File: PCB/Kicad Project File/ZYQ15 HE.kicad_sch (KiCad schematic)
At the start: 130 parts, among them J1 I2C OLED, U16 ESP32-S3-DevKitC

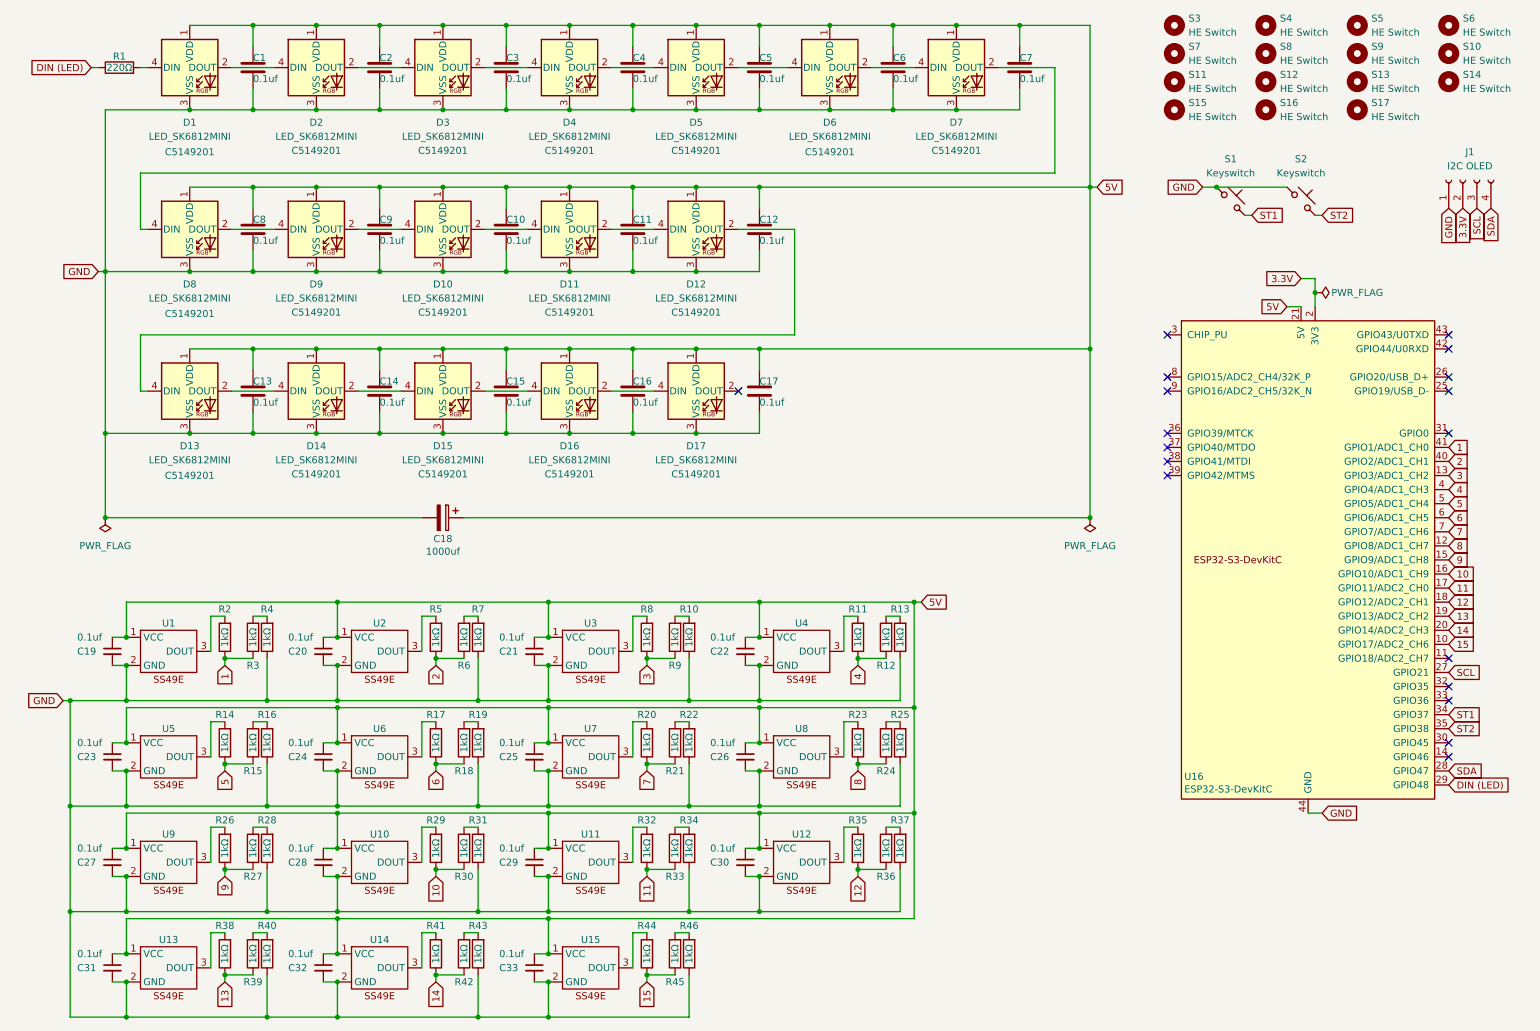
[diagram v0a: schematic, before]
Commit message: Updated PCB design files
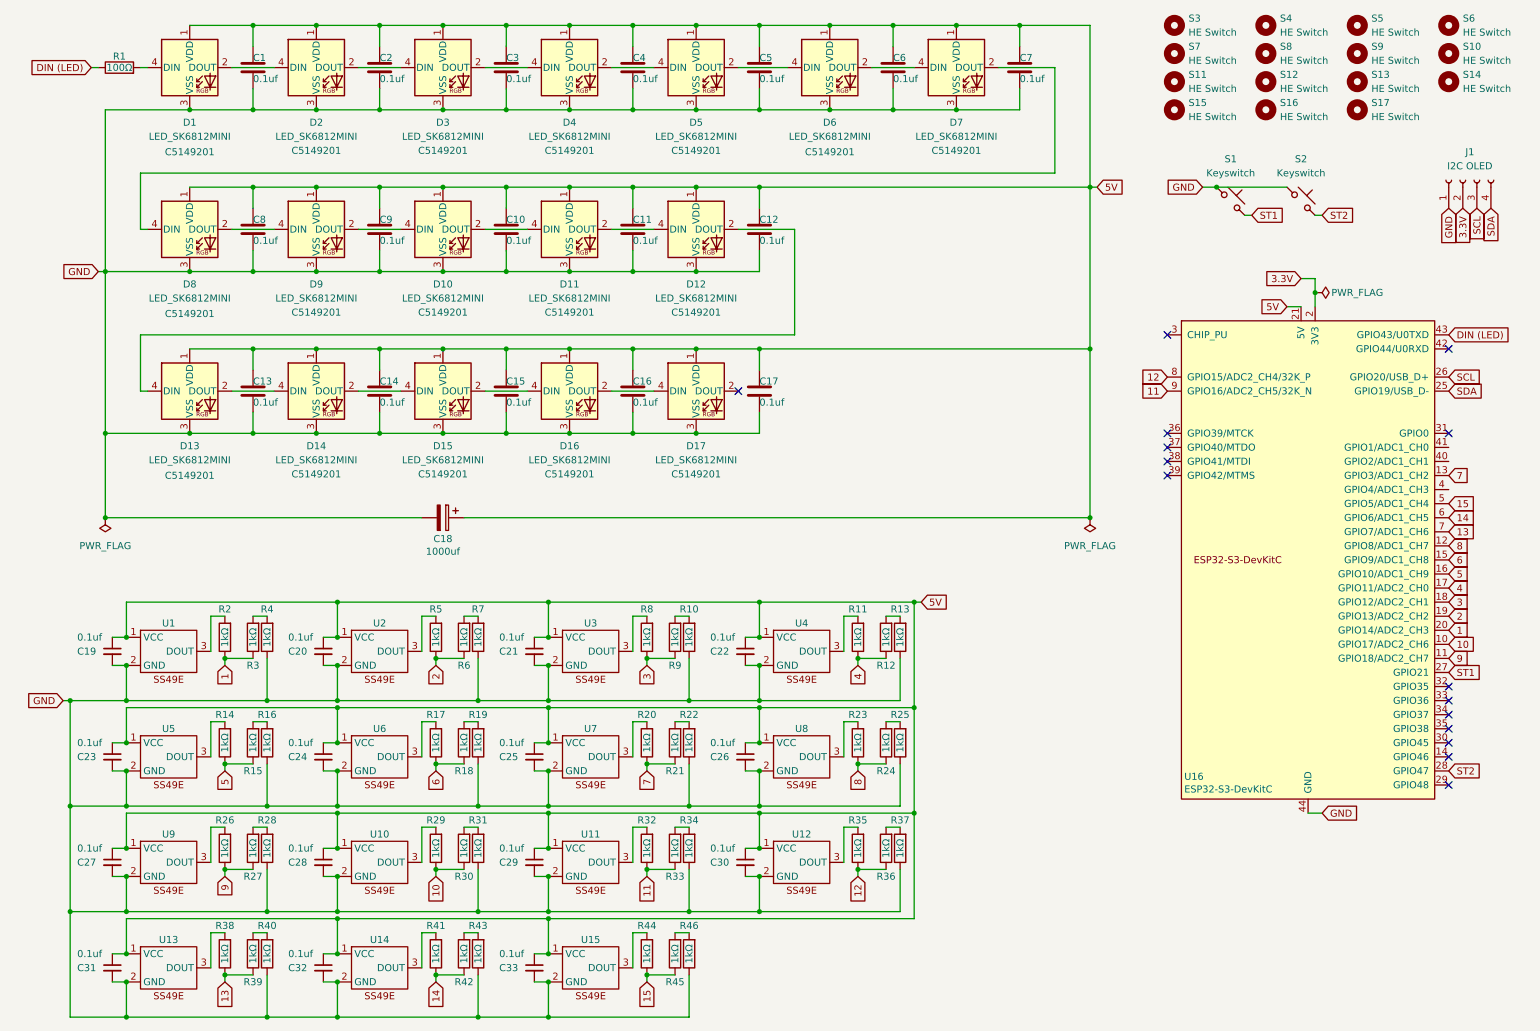
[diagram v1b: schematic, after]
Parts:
- C18: footprint Capacitor_THT:CP_Radial_D10.0mm_P5.00mm -> Capacitor_THT:CP_Radial_D10.0mm_P5.00mm_BACK
- R1: value 220Ω -> 100Ω
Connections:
- net 1: now also U16.20 (GPIO14/ADC2_CH3); no longer U16.41 (GPIO1/ADC1_CH0)
- net 10: now also U16.10 (GPIO17/ADC2_CH6); no longer U16.16 (GPIO10/ADC1_CH9)
- net 11: now also U16.9 (GPIO16/ADC2_CH5/32K_N); no longer U16.17 (GPIO11/ADC2_CH0)
- net 12: now also U16.8 (GPIO15/ADC2_CH4/32K_P); no longer U16.18 (GPIO12/ADC2_CH1)
- net 13: now also U16.7 (GPIO7/ADC1_CH6); no longer U16.19 (GPIO13/ADC2_CH2)
- net 14: now also U16.6 (GPIO6/ADC1_CH5); no longer U16.20 (GPIO14/ADC2_CH3)
- net 15: now also U16.5 (GPIO5/ADC1_CH4); no longer U16.10 (GPIO17/ADC2_CH6)
- net 2: now also U16.19 (GPIO13/ADC2_CH2); no longer U16.40 (GPIO2/ADC1_CH1)
- net 3: now also U16.18 (GPIO12/ADC2_CH1); no longer U16.13 (GPIO3/ADC1_CH2)
- net 4: now also U16.17 (GPIO11/ADC2_CH0); no longer U16.4 (GPIO4/ADC1_CH3)
- net 5: now also U16.16 (GPIO10/ADC1_CH9); no longer U16.5 (GPIO5/ADC1_CH4)
- net 6: now also U16.15 (GPIO9/ADC1_CH8); no longer U16.6 (GPIO6/ADC1_CH5)
- net 7: now also U16.13 (GPIO3/ADC1_CH2); no longer U16.7 (GPIO7/ADC1_CH6)
- net 9: now also U16.11 (GPIO18/ADC2_CH7); no longer U16.15 (GPIO9/ADC1_CH8)
- net DIN (LED): now also U16.43 (GPIO43/U0TXD); no longer U16.29 (GPIO48)
- net SCL: now also U16.26 (GPIO20/USB_D+); no longer U16.27 (GPIO21)
- net SDA: now also U16.25 (GPIO19/USB_D-); no longer U16.28 (GPIO47)
- net ST1: now also U16.27 (GPIO21); no longer U16.34 (GPIO37)
- net ST2: now also U16.28 (GPIO47); no longer U16.35 (GPIO38)
- no-connect marks 18 -> 15
